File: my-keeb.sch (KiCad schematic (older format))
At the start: 108 parts, among them SW1 SW_Push, U1 ATmega32U4-AU, Y1 16MHz

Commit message: Finished schema
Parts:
- F1: footprint (none) -> Fuse:Fuse_1206_3216Metric
- MX1, MX10, MX11, MX12, MX13, MX14, MX15, MX16, MX17, MX18, MX19, MX2, MX20, MX21, MX22, MX24, MX25, MX26, MX27, MX29, MX3, MX30, MX31, MX32, MX33, MX34, MX35, MX36, MX37, MX38, MX39, MX4, MX40, MX41, MX42, MX43, MX44, MX45, MX46, MX5, MX6, MX7, MX8, MX9: footprint (none) -> MX_Alps_Hybrid:MX-1U-NoLED
- MX23, MX28: footprint (none) -> MX_Alps_Hybrid:MX-1.5U-NoLED
- R1, R2, R3, R4: footprint (none) -> Resistor_SMD:R_0805_2012Metric
- SW1: footprint (none) -> random-keyboard-parts:SKQG-1155865
- USB1: footprint (none) -> random-keyboard-parts:Molex-0548190589
- Y1: footprint (none) -> Crystal:Crystal_SMD_3225-4Pin_3.2x2.5mm

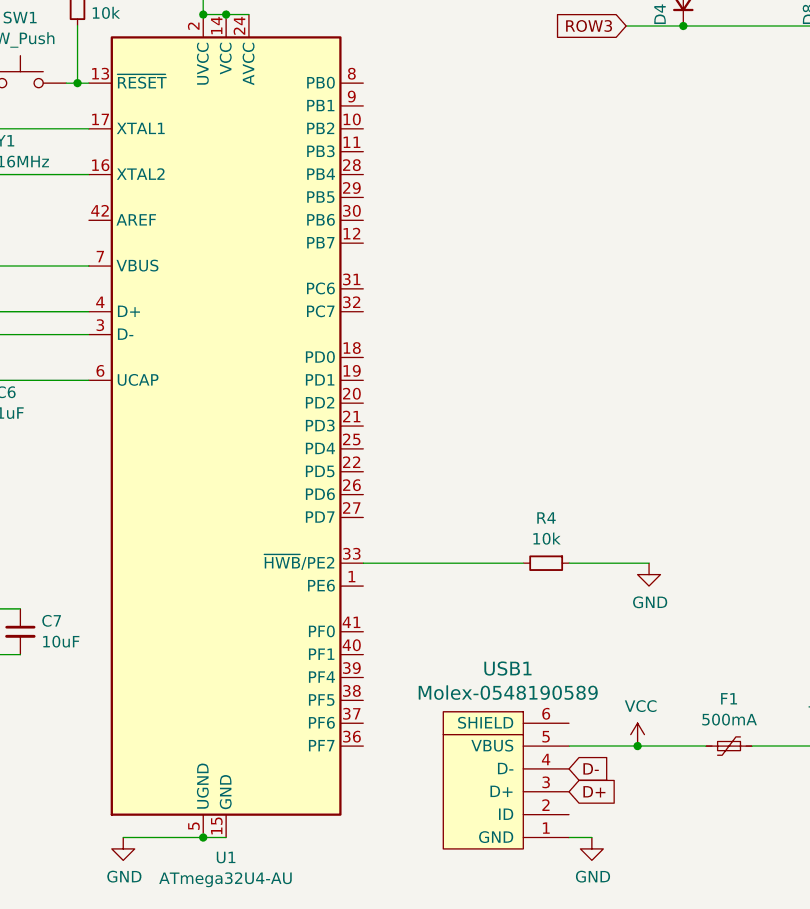
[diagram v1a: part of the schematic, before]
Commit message: Working on matrix
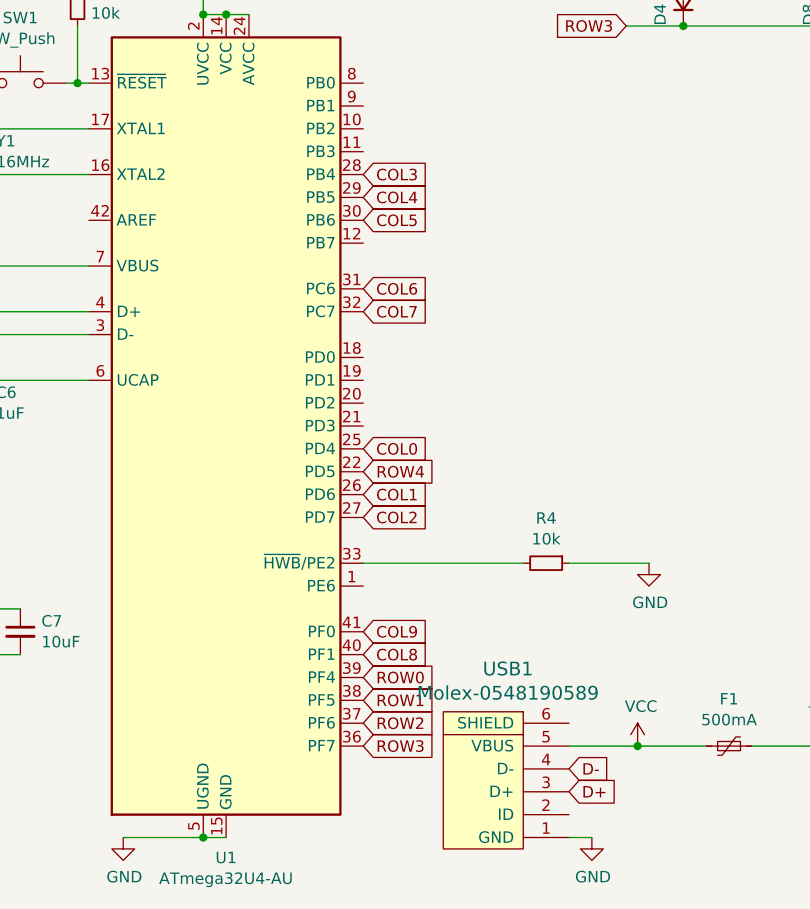
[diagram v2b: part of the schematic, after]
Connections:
- net COL0: now also U1.25 (PD4)
- net COL1: now also U1.26 (PD6)
- net COL2: now also U1.27 (PD7)
- net COL3: now also U1.28 (PB4)
- net COL4: now also U1.29 (PB5)
- net COL5: now also U1.30 (PB6)
- net COL6: now also U1.31 (PC6)
- net COL7: now also U1.32 (PC7)
- net COL8: now also U1.40 (PF1)
- net COL9: now also U1.41 (PF0)
- net ROW0: now also U1.39 (PF4)
- net ROW1: now also U1.38 (PF5)
- net ROW2: now also U1.37 (PF6)
- net ROW3: now also U1.36 (PF7)
- net ROW4: now also U1.22 (PD5)
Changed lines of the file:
@@
 Text GLabel 10900 1000 1    50   Input ~ 0
 COL9
+Text GLabel 3350 7100 2    50   Input ~ 0
+ROW3
+Text GLabel 3350 7000 2    50   Input ~ 0
+ROW2
+Text GLabel 3350 6900 2    50   Input ~ 0
+ROW1
+Text GLabel 3350 6800 2    50   Input ~ 0
+ROW0
+Text GLabel 3350 5900 2    50   Input ~ 0
+ROW4
+Text GLabel 3350 5200 2    50   Input ~ 0
+COL7
+Text GLabel 3350 6700 2    50   Input ~ 0
+COL8
+Text GLabel 3350 5100 2    50   Input ~ 0
+COL6
+Text GLabel 3350 4800 2    50   Input ~ 0
+COL5
+Text GLabel 3350 4700 2    50   Input ~ 0
+COL4
+Text GLabel 3350 4600 2    50   Input ~ 0
+COL3
+Text GLabel 3350 6100 2    50   Input ~ 0
+COL2
+Text GLabel 3350 6000 2    50   Input ~ 0
+COL1
+Text GLabel 3350 5800 2    50   Input ~ 0
+COL0
+Text GLabel 3350 6600 2    50   Input ~ 0
+COL9
 $EndSCHEMATC
